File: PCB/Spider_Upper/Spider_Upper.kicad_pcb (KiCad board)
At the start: 2 copper layers, 63 x 63 mm, 21 parts, among them J1 Conn_02x06_Odd_Even, J2 Conn_02x06_Odd_Even, J3 Conn_02x06_Odd_Even, J4 Conn_02x06_Odd_Even, J5 Conn_01x02, U3 LM2675M-5

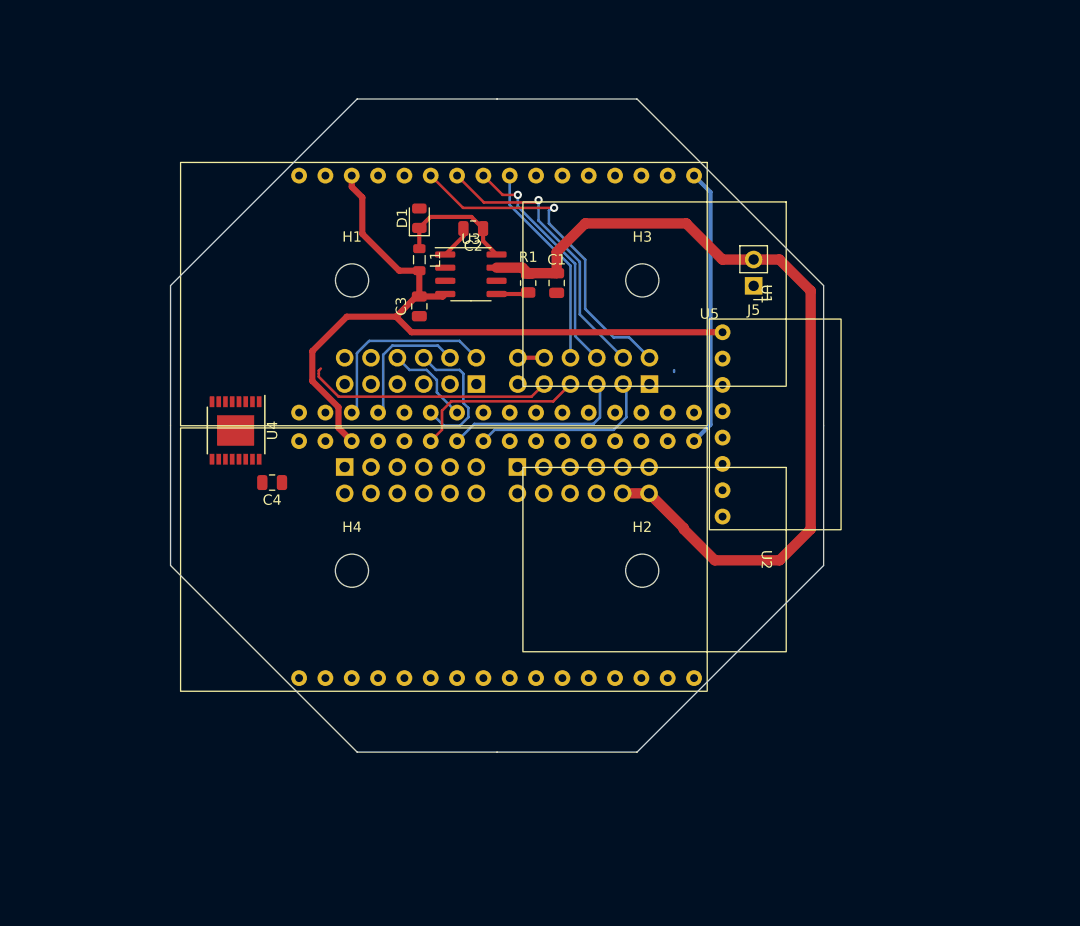
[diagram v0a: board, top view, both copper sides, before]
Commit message: finished V1 PCB
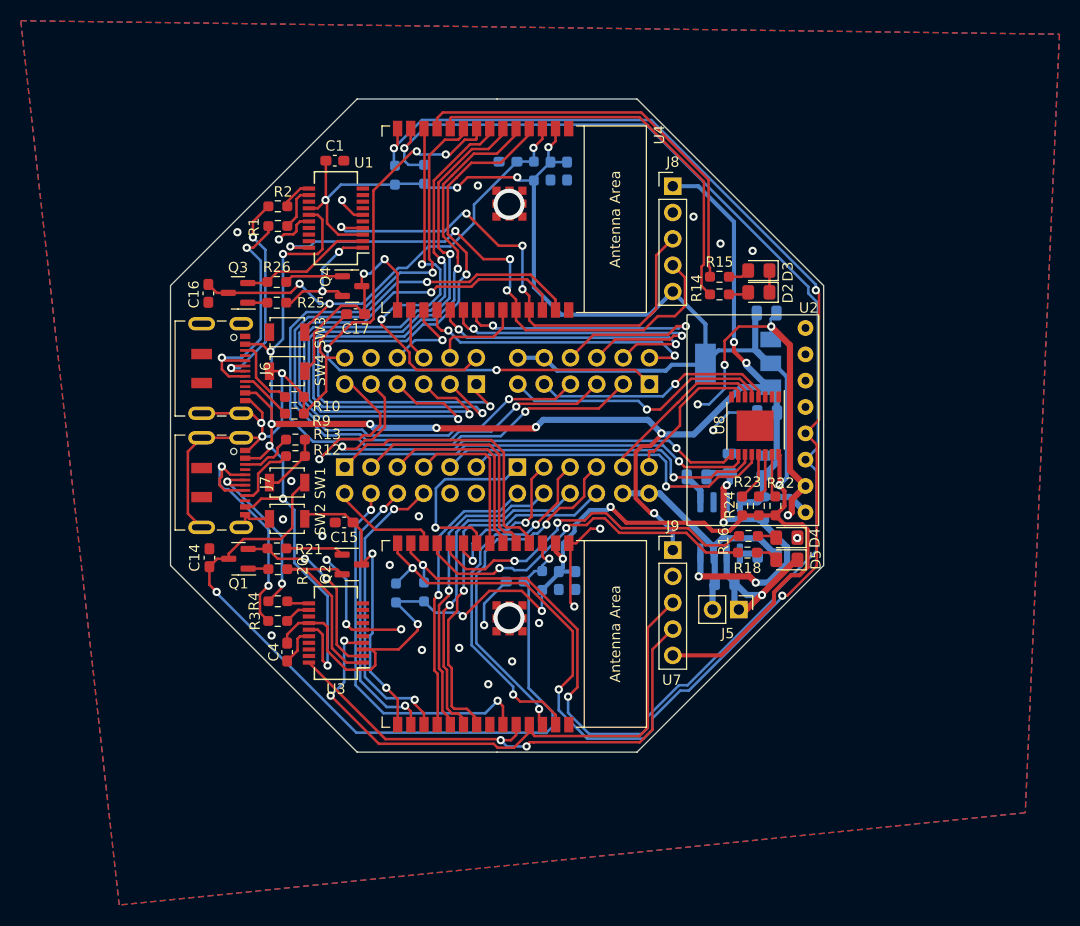
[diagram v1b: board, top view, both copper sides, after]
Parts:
- removed H1, H2, H3, H4: MountingHole, MountingHole:MountingHole_3.2mm_M3
- removed the U2 at (111.0, 107.7)
- added C10: 0.1u, Capacitor_SMD:C_0603_1608Metric_Pad1.08x0.95mm_HandSolder, B.Cu at (98.3, 109.7)
- added C11: 100nF, Capacitor_SMD:C_0805_2012Metric, B.Cu at (116.8, 93.5)
- added C12: 0.1u, Capacitor_SMD:C_0603_1608Metric_Pad1.08x0.95mm_HandSolder, B.Cu at (92.5, 109.8)
- added C13: 10uF, Capacitor_SMD:C_0805_2012Metric, B.Cu at (116.8, 83.9)
- added C14: 0.1u, Capacitor_SMD:C_0603_1608Metric_Pad1.08x0.95mm_HandSolder, F.Cu at (63.0, 107.5)
- added C15: 0.1u, Capacitor_SMD:C_0603_1608Metric_Pad1.08x0.95mm_HandSolder, F.Cu at (76.0, 104.1)
- added C16: 0.1u, Capacitor_SMD:C_0603_1608Metric_Pad1.08x0.95mm_HandSolder, F.Cu at (62.9, 82.0)
- added C17: 0.1u, Capacitor_SMD:C_0603_1608Metric_Pad1.08x0.95mm_HandSolder, F.Cu at (77.1, 84.0)
- added C5: 0.1u, Capacitor_SMD:C_0603_1608Metric_Pad1.08x0.95mm_HandSolder, B.Cu at (91.8, 69.3)
- added C6: 100uF, Capacitor_SMD:C_0805_2012Metric, B.Cu at (112.7, 109.9)
- added C7: 10nF, Capacitor_SMD:C_0805_2012Metric, B.Cu at (110.0, 99.7)
- added C8: 68uF, Capacitor_SMD:C_0805_2012Metric, B.Cu at (116.5, 98.6)
- added C9: 10u, Capacitor_SMD:C_0603_1608Metric_Pad1.08x0.95mm_HandSolder, B.Cu at (96.7, 109.7)
- added D2: LED, LED_SMD:LED_0805_2012Metric_Pad1.15x1.40mm_HandSolder, F.Cu at (116.0, 81.9)
- added D3: LED, LED_SMD:LED_0805_2012Metric_Pad1.15x1.40mm_HandSolder, F.Cu at (116.0, 79.8)
- added D4: LED, LED_SMD:LED_0805_2012Metric_Pad1.15x1.40mm_HandSolder, F.Cu at (118.7, 105.6)
- added D5: LED, LED_SMD:LED_0805_2012Metric_Pad1.15x1.40mm_HandSolder, F.Cu at (118.7, 107.7)
- added J6: USB_C_Receptacle_USB2.0, Connector_USB:USB_C_Receptacle_JAE_DX07S016JA1R1500, F.Cu at (63.4, 89.2)
- added J7: USB_C_Receptacle_USB2.0, Connector_USB:USB_C_Receptacle_JAE_DX07S016JA1R1500, F.Cu at (63.4, 100.2)
- added J8: Conn_01x05, Connector_PinHeader_2.54mm:PinHeader_1x05_P2.54mm_Vertical, F.Cu at (107.7, 71.7)
- added J9: Conn_01x05, Connector_PinHeader_2.54mm:PinHeader_1x05_P2.54mm_Vertical, F.Cu at (107.7, 106.8)
- added Q1: DNBT8105-7, Package_TO_SOT_SMD:SOT-23, F.Cu at (65.8, 107.6)
- added Q2: DNBT8105-7, Package_TO_SOT_SMD:SOT-23, F.Cu at (76.7, 108.2)
- added Q3: DNBT8105-7, Package_TO_SOT_SMD:SOT-23, F.Cu at (65.8, 82.0)
- added Q4: DNBT8105-7, Package_TO_SOT_SMD:SOT-23, F.Cu at (76.8, 81.3)
- added R10: 5.1k, Resistor_SMD:R_0603_1608Metric_Pad0.98x0.95mm_HandSolder, F.Cu at (71.2, 92.0)
- added R11: 10k, Resistor_SMD:R_0603_1608Metric_Pad0.98x0.95mm_HandSolder, B.Cu at (95.1, 109.7)
- added R12: 5.1k, Resistor_SMD:R_0603_1608Metric_Pad0.98x0.95mm_HandSolder, F.Cu at (71.3, 97.7)
- added R13: 5.1k, Resistor_SMD:R_0603_1608Metric_Pad0.98x0.95mm_HandSolder, F.Cu at (71.3, 96.1)
- added R14: 280, Resistor_SMD:R_0603_1608Metric_Pad0.98x0.95mm_HandSolder, F.Cu at (112.2, 82.1)
- added R15: 280, Resistor_SMD:R_0603_1608Metric_Pad0.98x0.95mm_HandSolder, F.Cu at (112.2, 80.4)
- added R16: 280, Resistor_SMD:R_0603_1608Metric_Pad0.98x0.95mm_HandSolder, F.Cu at (115.0, 105.4)
- added R17: 2.2k, Resistor_SMD:R_0603_1608Metric_Pad0.98x0.95mm_HandSolder, B.Cu at (81.0, 110.9)
- added R18: 180, Resistor_SMD:R_0603_1608Metric_Pad0.98x0.95mm_HandSolder, F.Cu at (114.9, 107.0)
- added R19: 2.2k, Resistor_SMD:R_0603_1608Metric_Pad0.98x0.95mm_HandSolder, B.Cu at (83.7, 110.8)
- added R2: 27, Resistor_SMD:R_0603_1608Metric_Pad0.98x0.95mm_HandSolder, F.Cu at (69.6, 73.6)
- added R20: 10k, Resistor_SMD:R_0603_1608Metric_Pad0.98x0.95mm_HandSolder, F.Cu at (69.6, 108.6)
- added R21: 10k, Resistor_SMD:R_0603_1608Metric_Pad0.98x0.95mm_HandSolder, F.Cu at (69.5, 106.6)
- added R22: 2.2k, Resistor_SMD:R_0603_1608Metric_Pad0.98x0.95mm_HandSolder, F.Cu at (117.6, 102.5)
- added R23: 2.2k, Resistor_SMD:R_0603_1608Metric_Pad0.98x0.95mm_HandSolder, F.Cu at (116.0, 102.5)
- added R24: 2.2k, Resistor_SMD:R_0603_1608Metric_Pad0.98x0.95mm_HandSolder, F.Cu at (114.4, 102.5)
- added R25: 10k, Resistor_SMD:R_0603_1608Metric_Pad0.98x0.95mm_HandSolder, F.Cu at (69.5, 82.9)
- added R26: 10k, Resistor_SMD:R_0603_1608Metric_Pad0.98x0.95mm_HandSolder, F.Cu at (69.5, 80.9)
- added R3: 27, Resistor_SMD:R_0603_1608Metric_Pad0.98x0.95mm_HandSolder, F.Cu at (69.6, 113.6)
- added R4: 27, Resistor_SMD:R_0603_1608Metric_Pad0.98x0.95mm_HandSolder, F.Cu at (69.6, 111.7)
- added R5: 10k, Resistor_SMD:R_0603_1608Metric_Pad0.98x0.95mm_HandSolder, B.Cu at (94.3, 70.2)
- added R6: 5k, Resistor_SMD:R_0805_2012Metric, B.Cu at (116.8, 107.3)
- added R7: 2.2k, Resistor_SMD:R_0603_1608Metric_Pad0.98x0.95mm_HandSolder, B.Cu at (80.9, 70.6)
- added R8: 2.2k, Resistor_SMD:R_0603_1608Metric_Pad0.98x0.95mm_HandSolder, B.Cu at (83.7, 70.5)
- added R9: 5.1k, Resistor_SMD:R_0603_1608Metric_Pad0.98x0.95mm_HandSolder, F.Cu at (71.2, 93.6)
- added SW1: SW_SPST, Button_Switch_SMD:SW_SPST_B3U-1000P, F.Cu at (70.5, 100.2)
- added SW2: SW_SPST, Button_Switch_SMD:SW_SPST_B3U-1000P, F.Cu at (70.5, 103.8)
- added SW3: SW_SPST, Button_Switch_SMD:SW_SPST_B3U-1000P, F.Cu at (70.5, 85.8)
- added SW4: SW_SPST, Button_Switch_SMD:SW_SPST_B3U-1000P, F.Cu at (70.5, 89.5)
- added U5: LM2675M-5, Package_SO:SOIC-8_3.9x4.9mm_P1.27mm, B.Cu at (112.3, 104.6)
- added U6: LD1117S33TR_SOT223, Package_TO_SOT_SMD:SOT-223-3_TabPin2, B.Cu at (114.0, 88.8)
- added U7: ESP32-C6-WROOM-1, Espressif:ESP32-C6-WROOM-1, F.Cu at (89.4, 114.8)
- added U8: ~, Package_SO:TSSOP-16-1EP_4.4x5mm_P0.65mm, F.Cu at (115.6, 94.8)
- C1: value 100uF -> 0.1u; footprint Capacitor_SMD:C_0805_2012Metric -> Capacitor_SMD:C_0603_1608Metric_Pad1.08x0.95mm_HandSolder
- C2: value 10nF -> 10u; footprint Capacitor_SMD:C_0805_2012Metric -> Capacitor_SMD:C_0603_1608Metric_Pad1.08x0.95mm_HandSolder; moved to B.Cu
- C3: value 68uF -> 0.1u; footprint Capacitor_SMD:C_0805_2012Metric -> Capacitor_SMD:C_0603_1608Metric_Pad1.08x0.95mm_HandSolder; moved to B.Cu
- C4: value 10uF -> 0.1u; footprint Capacitor_SMD:C_0805_2012Metric -> Capacitor_SMD:C_0603_1608Metric_Pad1.08x0.95mm_HandSolder
- D1, L1: moved to B.Cu
- R1: value 5k -> 27; footprint Resistor_SMD:R_0805_2012Metric -> Resistor_SMD:R_0603_1608Metric_Pad0.98x0.95mm_HandSolder
- U1: value ~ -> FT231XS; footprint Adafruit ESPs:ESP32-C6 -> Package_SO:SSOP-20_3.9x8.7mm_P0.635mm
- U3: value LM2675M-5 -> FT231XS; footprint Package_SO:SOIC-8_3.9x4.9mm_P1.27mm -> Package_SO:SSOP-20_3.9x8.7mm_P0.635mm
- U4: value ~ -> ESP32-C6-WROOM-1; footprint Package_SO:TSSOP-16-1EP_4.4x5mm_P0.65mm -> Espressif:ESP32-C6-WROOM-1
- moved L1 40.9 mm to (116.4, 102.7), turned to 90 degrees
- moved D1 38.2 mm to (113.2, 98.4)
- moved U3 37.0 mm to (75.2, 114.8), turned to 180 degrees
- moved U1 36.6 mm to (75.2, 74.7), turned to 180 degrees
- moved U4 31.4 mm to (89.4, 74.8)
- moved J5 31.3 mm to (114.1, 112.5), turned to -90 degrees
- moved R1 24.8 mm to (69.6, 75.5), turned to 0 degrees
- moved C1 24.4 mm to (75.1, 69.2), turned to 0 degrees
- moved U2 22.5 mm to (121.8, 104.4), turned to 180 degrees
- moved C3 19.3 mm to (97.5, 70.2)
- moved C4 16.4 mm to (70.5, 116.6), turned to -90 degrees
- moved C2 9.29 mm to (95.9, 70.2), turned to -90 degrees
- renumbered U5 to U2
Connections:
- C1 pad 1: +12V -> +3.3V
- C2 pad 1: Net-(D1-K) -> +3.3V
- C2 pad 2: Net-(U3-CB) -> GND
- C3 pad 1: +5V -> +3.3V
- C4 pad 1: GND -> +3.3V
- C4 pad 2: +5V -> GND
- R1 pad 1: +12V -> /USB_DM0
- R1 pad 2: Net-(U3-ON/~{OFF}) -> Net-(U1-USBDM)
- U3 pad 1: Net-(U3-CB) -> /DTR1
- U3 pad 2: unconnected-(U3-NC-Pad2) -> /RTS1
- U3 pad 3: unconnected-(U3-NC-Pad3) -> +3.3V
- U3 pad 4: +5V -> /TX1
- U3 pad 5: Net-(U3-ON/~{OFF}) -> unconnected-(U3-~{RI}-Pad5)
- U3 pad 7: +12V -> unconnected-(U3-~{DSR}-Pad7)
- U3 pad 8: Net-(D1-K) -> unconnected-(U3-~{DCD}-Pad8)
- U4 pad 1: /SW_20 -> GND
- U4 pad 10: /GPIO15 -> /LED00
- U4 pad 11: /GPIO23 -> /LED01
- U4 pad 12: /SW_11 -> /EA_20
- U4 pad 13: /SW_00 -> /SCL
- U4 pad 14: /SW_01 -> /SDA
- U4 pad 15: /SW_10 -> /BOOT0
- U4 pad 16: +5V -> /EA_21
- U4 pad 17: (no net) -> /EB_21
- U4 pad 2: /SW_30 -> +3.3V
- U4 pad 3: /GPIO22 -> /EN0
- U4 pad 4: /SW_31 -> /INA_20
- U4 pad 5: /SW_21 -> /INB_20
- U4 pad 6: GND -> /INA_21
- U4 pad 7: GND -> /INB_21
- U4 pad 8: GND -> /INA_00
- U4 pad 9: /GPIO17 -> /INB_00
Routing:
- net +3.3V: track 29.5 -> 227.0 mm, vias 0 -> 10
- net GND: track 0.00 -> 164.0 mm, vias 0 -> 36
- net /SDA: track 0.00 -> 145.5 mm, vias 0 -> 5
- net /SCL: track 0.00 -> 142.0 mm, vias 0 -> 3
- net +5V: track 73.0 -> 179.4 mm, vias 0 -> 13
- net /EN1: track 0.00 -> 76.5 mm, vias 0 -> 2
- net /INA_00: track 0.00 -> 64.6 mm, vias 0 -> 4
- net /INB_21: track 0.00 -> 63.8 mm, vias 0 -> 2
- net /INA_21: track 0.00 -> 63.7 mm, vias 0 -> 2
- net /INB_20: track 0.00 -> 63.4 mm, vias 0 -> 2
- net /INA_20: track 0.47 -> 62.8 mm, vias 0 -> 2
- net /INB_00: track 18.1 -> 76.6 mm, vias 0 -> 2
- net +12V: track 81.6 -> 25.0 mm
- net /TX1: track 0.00 -> 55.9 mm, vias 0 -> 2
- net /SW_21: track 0.00 -> 55.8 mm, vias 0 -> 2
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- added copper zone on B.Cu, net GND
- added copper zone on F.Cu, net GND
